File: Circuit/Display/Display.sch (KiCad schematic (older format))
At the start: 29 parts, among them J1 Conn_PIC_ICSP_ICD, J2 Conn_01x04_Male, U1 TBD62783A, U2 PIC16F18854-SO, U3 ULN2803A

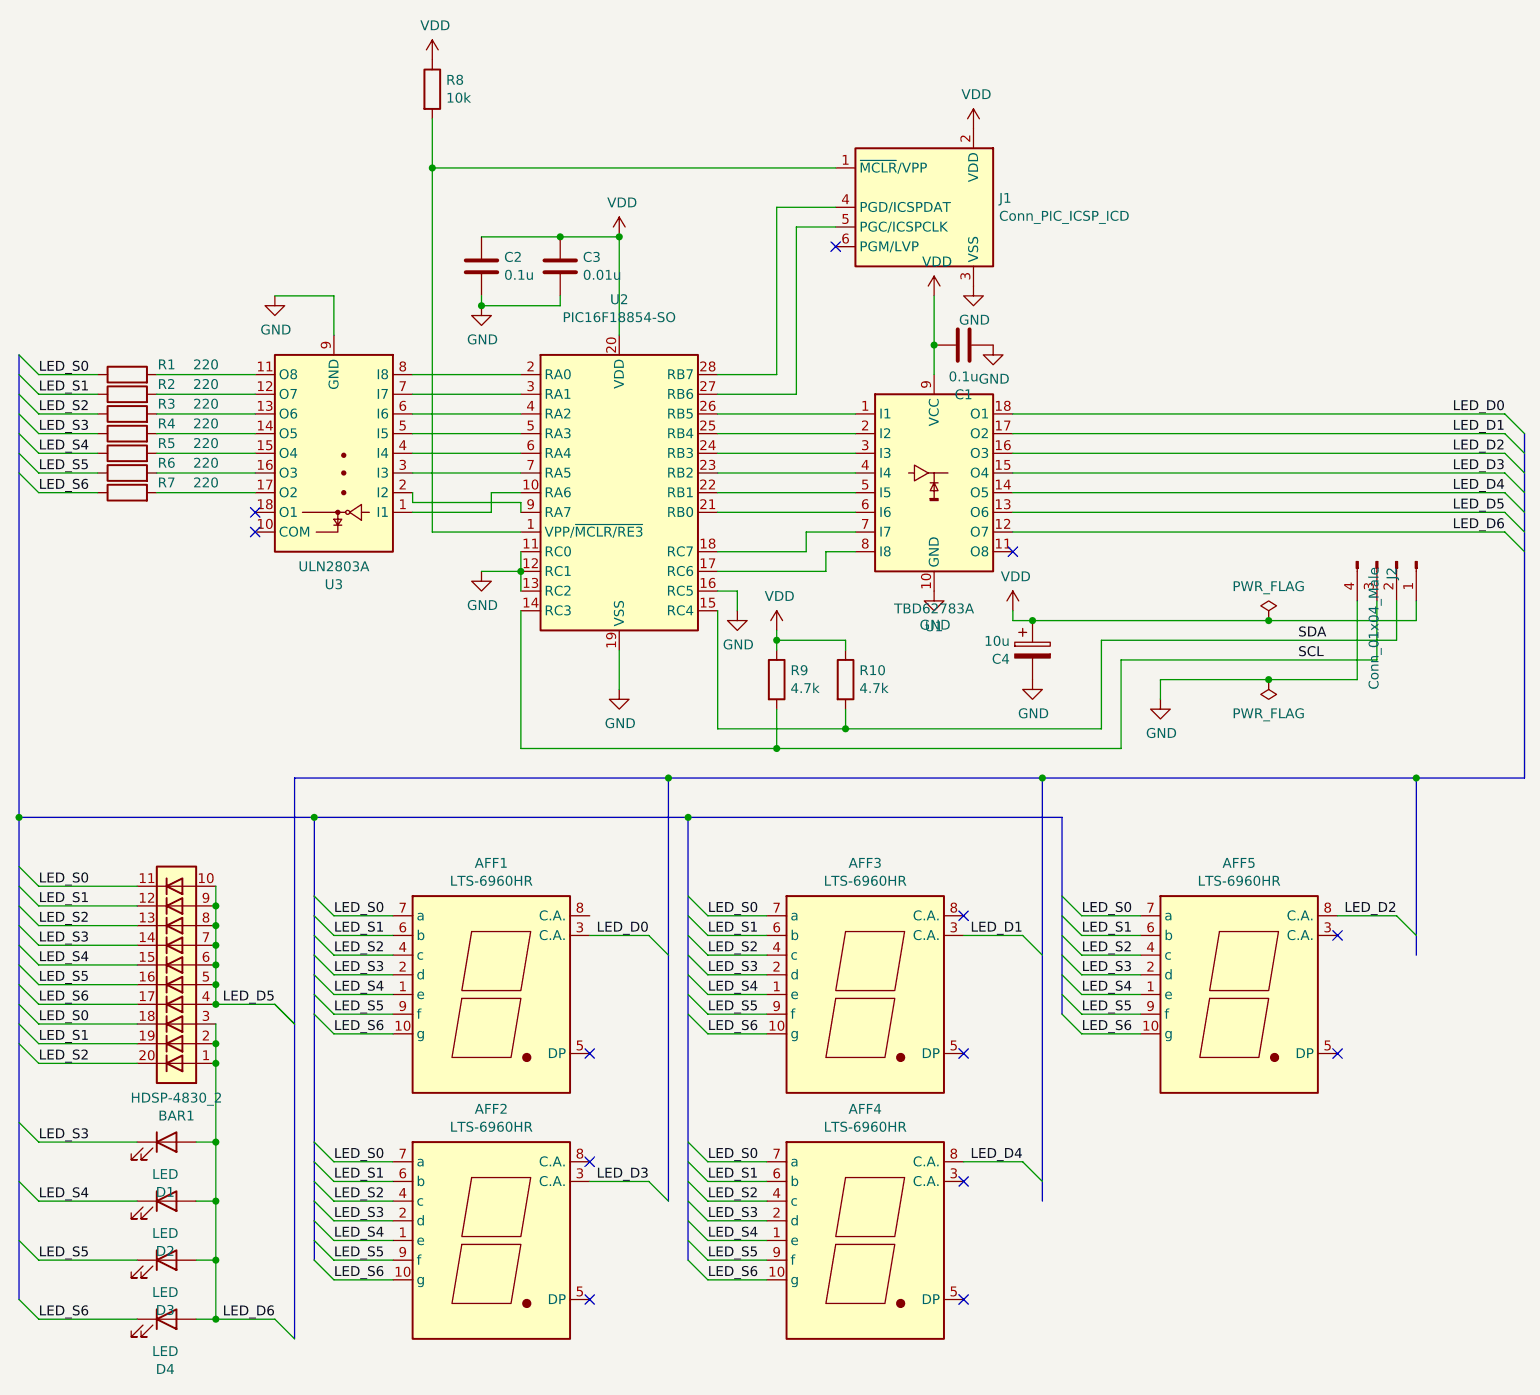
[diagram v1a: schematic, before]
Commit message: メイン飛んだ
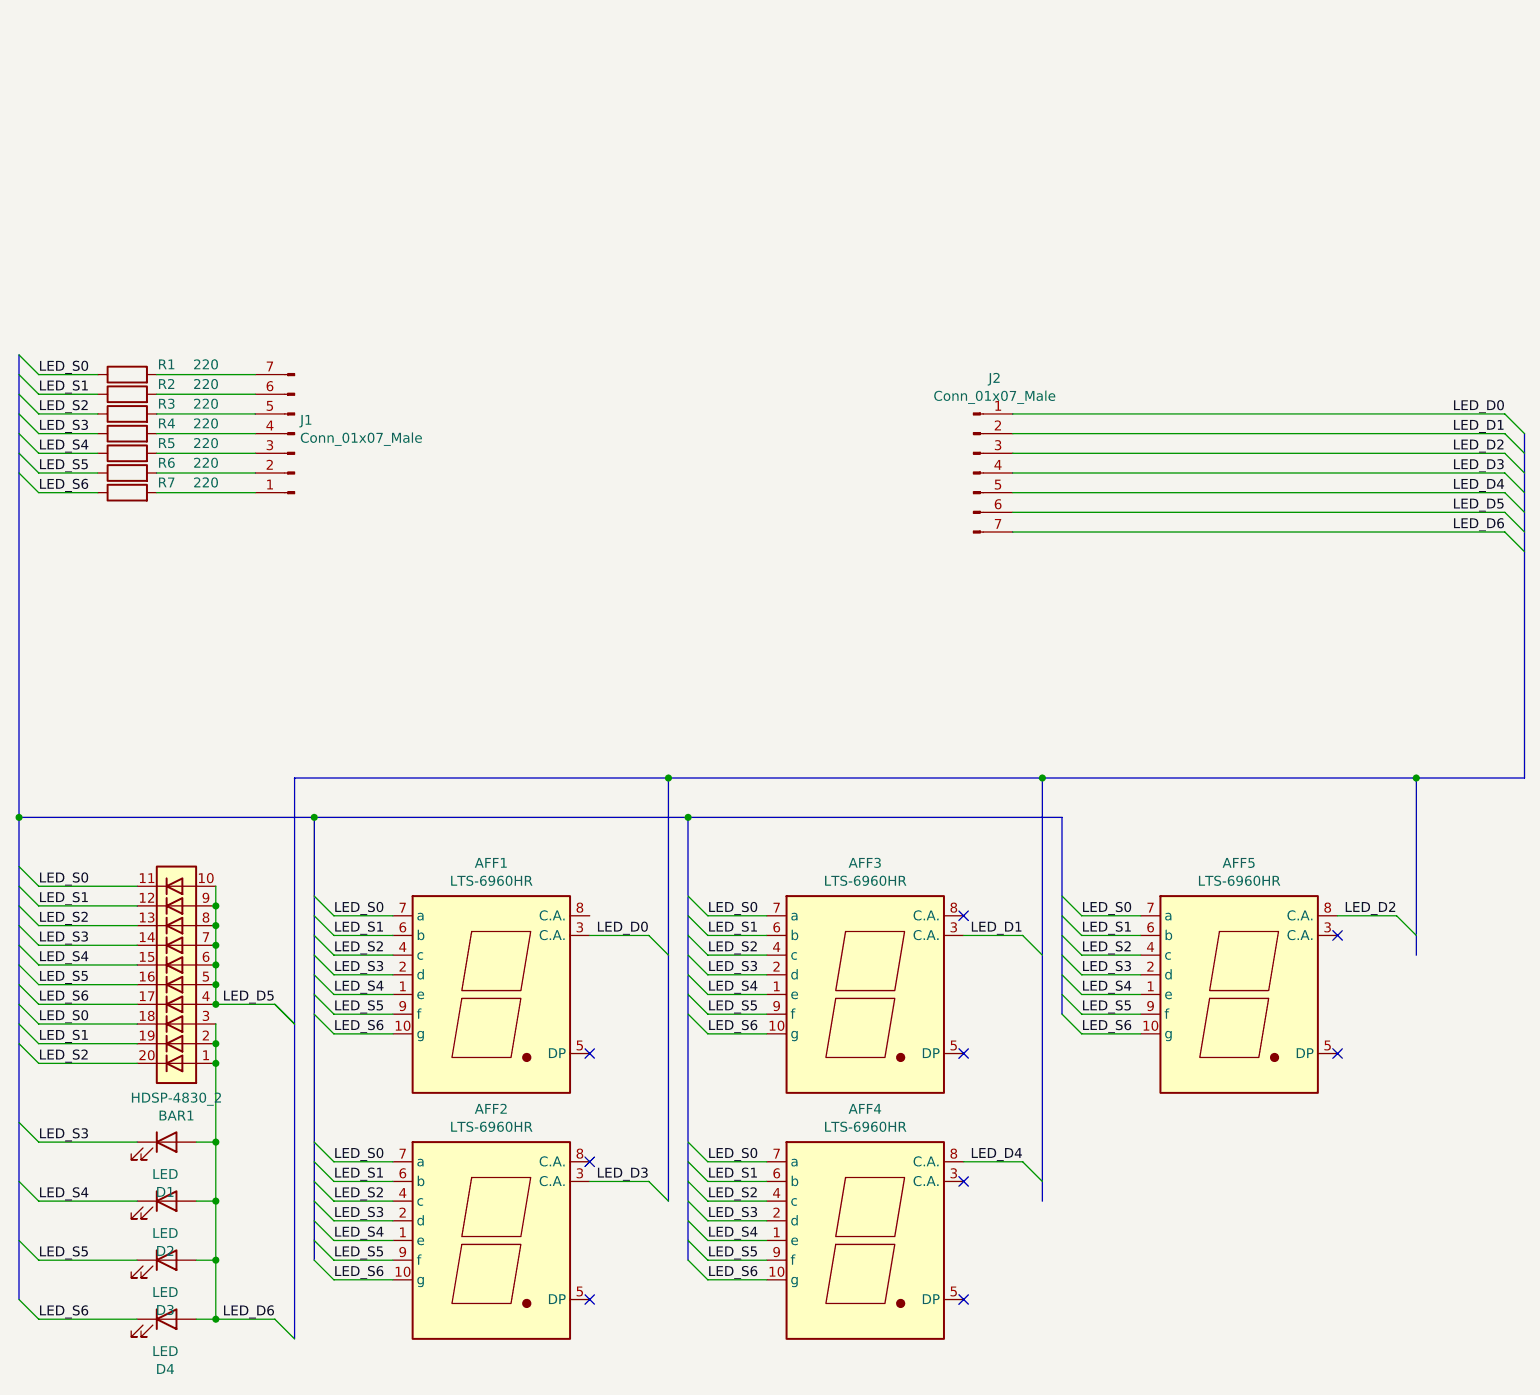
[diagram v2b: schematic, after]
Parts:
- removed C1, C2: 0.1u, Capacitor_THT:C_Disc_D3.0mm_W1.6mm_P2.50mm, symbol Device:C
- removed C3: 0.01u, Capacitor_THT:C_Disc_D3.0mm_W2.0mm_P2.50mm, symbol Device:C
- removed C4: 10u, Capacitor_THT:CP_Radial_D5.0mm_P2.50mm, symbol Device:CP
- removed J1: Conn_PIC_ICSP_ICD, Connector_PinHeader_2.54mm:PinHeader_1x06_P2.54mm_Horizontal, symbol Connector:Conn_PIC_ICSP_ICD
- removed J2: Conn_01x04_Male, Connector_PinHeader_2.54mm:PinHeader_1x04_P2.54mm_Horizontal, symbol Connector:Conn_01x04_Male
- removed R10, R9: 4.7k, Resistor_THT:R_Axial_DIN0204_L3.6mm_D1.6mm_P7.62mm_Horizontal, symbol Device:R
- removed R8: 10k, Resistor_THT:R_Axial_DIN0204_L3.6mm_D1.6mm_P7.62mm_Horizontal, symbol Device:R
- removed U1: TBD62783A, Package_DIP:DIP-18_W7.62mm, symbol Transistor_Array:TBD62783A
- removed U2: PIC16F18854-SO, Package_DIP:DIP-28_W7.62mm, symbol MCU_Microchip_PIC16:PIC16F18854-SO
- removed U3: ULN2803A, Package_DIP:DIP-18_W7.62mm, symbol Transistor_Array:ULN2803A
- added J1, J2: Conn_01x07_Male, Connector_PinHeader_2.54mm:PinHeader_1x07_P2.54mm_Vertical, symbol Connector:Conn_01x07_Male
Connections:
- net LED_D0: now also J2.1 (Pin_1)
- net LED_D1: now also J2.2 (Pin_2)
- net LED_D2: now also J2.3 (Pin_3)
- net LED_D3: now also J2.4 (Pin_4)
- net LED_D4: now also J2.5 (Pin_5)
- net LED_D5: now also J2.6 (Pin_6)
- net LED_D6: now also J2.7 (Pin_7)
- net at R1.2: now also J1.7 (Pin_7)
- net at R2.2: now also J1.6 (Pin_6)
- net at R3.2: now also J1.5 (Pin_5)
- net at R4.2: now also J1.4 (Pin_4)
- net at R5.2: now also J1.3 (Pin_3)
- net at R6.2: now also J1.2 (Pin_2)
- net at R7.2: now also J1.1 (Pin_1)
- no-connect marks 13 -> 9
